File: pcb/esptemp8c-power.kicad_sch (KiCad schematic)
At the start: 27 parts, among them J4 24VAC, J5 USB_C_Receptacle_USB2.0, U2 BD9G101G, U3 AMS1117-3.3

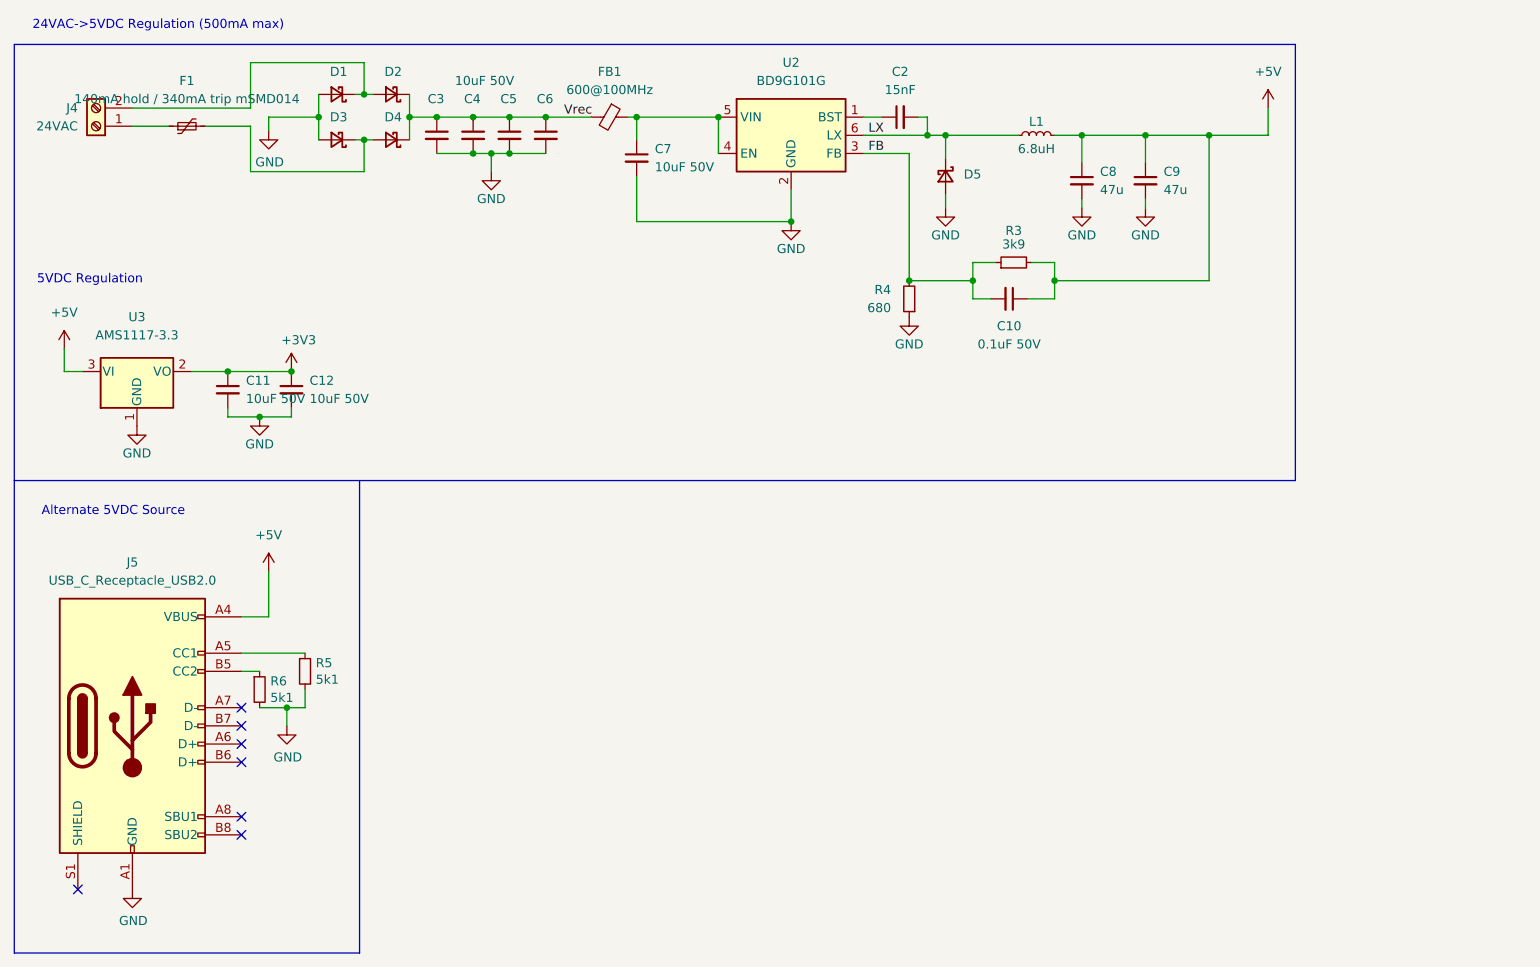
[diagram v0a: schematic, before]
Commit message: updates for v2
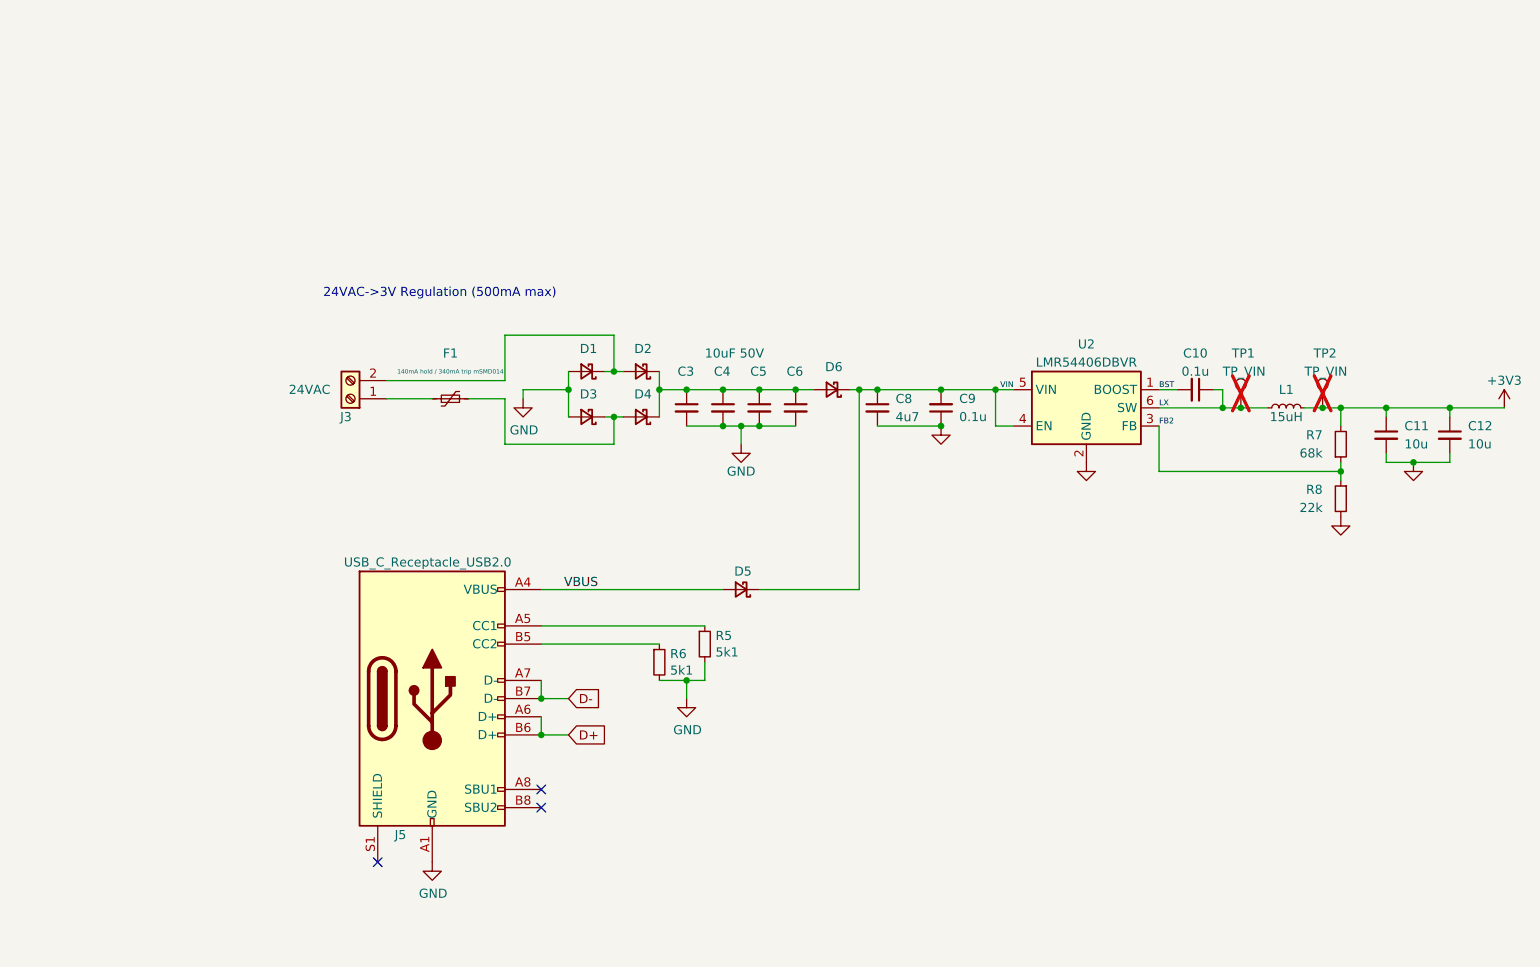
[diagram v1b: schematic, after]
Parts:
- removed C2: 15nF, Capacitor_SMD:C_0603_1608Metric, symbol Device:C_Small
- removed C7: 10uF 50V, Capacitor_SMD:C_1206_3216Metric, symbol Device:C_Small
- removed FB1: 600@100MHz, Inductor_SMD:L_0805_2012Metric, symbol Device:FerriteBead_Small
- removed J4: 24VAC, Connector_Phoenix_MSTB:PhoenixContact_MSTBA_2,5_2-G-5,08_1x02_P5.08mm_Horizontal, symbol Connector:Screw_Terminal_01x02
- removed R3: 3k9, Resistor_SMD:R_0402_1005Metric, symbol Device:R_Small
- removed R4: 680, Resistor_SMD:R_0402_1005Metric, symbol Device:R_Small
- removed U2: BD9G101G, Package_TO_SOT_SMD:SOT-23-6, symbol Regulator_Switching:AOZ1280CI
- removed U3: AMS1117-3.3, Package_TO_SOT_SMD:SOT-223-3_TabPin2, symbol Regulator_Linear:AP1117-33
- added D6: SS210, Diode_SMD:D_SMA, symbol Device:D_Schottky_Small
- added J3: 24VAC, Connector_Phoenix_MC:PhoenixContact_MC_1,5_2-G-3.81_1x02_P3.81mm_Horizontal, symbol Connector:Screw_Terminal_01x02
- added R7: 68k, Resistor_SMD:R_0402_1005Metric, symbol Device:R_Small
- added R8: 22k, Resistor_SMD:R_0402_1005Metric, symbol Device:R_Small
- added TP1, TP2: TP_VIN, Connector_PinHeader_2.54mm:PinHeader_1x01_P2.54mm_Vertical, symbol Connector:TestPoint
- added U2: LMR54406DBVR, Package_TO_SOT_SMD:TSOT-23-6, symbol Regulator_Switching:LM2840X
- C10: value 0.1uF 50V -> 0.1u
- C11, C12: value 10uF 50V -> 10u; footprint Capacitor_SMD:C_1206_3216Metric -> Capacitor_SMD:C_0805_2012Metric; LCSC C13585 -> C15850
- C8: value 47u -> 4u7; LCSC C96123 -> C29823
- C9: value 47u -> 0.1u; footprint Capacitor_SMD:C_1206_3216Metric -> Capacitor_SMD:C_0603_1608Metric; LCSC C96123 -> C14663
- D5: value SS210 -> CUS05S40.H3F; footprint Diode_SMD:D_SMA -> Diode_SMD:D_SOD-323; LCSC C14996 -> C2762696
- J5: symbol Connector:USB_C_Receptacle_USB2.0 -> Connector:USB_C_Receptacle_USB2.0_16P
- L1: value 6.8uH -> 15uH; footprint Inductor_SMD:L_Sunlord_SWPA60xxS -> Inductor_SMD:L_Sunlord_SWPA6028S; LCSC C57254 -> C83373; PN (none) -> SRN6045-150M or SWPA6045S150MT
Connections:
- net +3V3: now also L1.2, R7.2, TP2.1
- net GND: now also C9.1, R8.2, U2.2 (GND); no longer C9.2, D5.2 (A)
- net LX: now also C10.1, TP1.1, U2.6 (SW); no longer D5.1 (K)
- net D+: now reaches J5.A6 (D+)
- net D+: now also J5.B6 (D+)
- net D-: now reaches J5.A7 (D-)
- net D-: now also J5.B7 (D-)
- net at F1.1: now also J3.1 (Pin_1)
- net at D1.1 (K), D2.2 (A): now also J3.2 (Pin_2)
- net +5V renamed VBUS
- net VBUS: now also D5.2 (A); no longer C10.1, C8.1, C9.1, L1.2
- net FB renamed BST
- net BST: now also U2.1 (BOOST)
- net Vrec: no longer names the net of C3.1, C4.1, C5.1, C6.1, D2.1 (K), D4.1 (K)
- net Vrec: now also D6.2 (A)
- new net FB2: R7.1, R8.1, U2.3 (FB)
- new net VIN: C8.1, C9.2, D5.1 (K), D6.1 (K), U2.4 (EN), U2.5 (VIN)
- no-connect marks 7 -> 3
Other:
- note added: "24VAC->3V Regulation (500mA max)"
- note removed: "24VAC->5VDC Regulation (500mA max)"
- note removed: "5VDC Regulation"
- note removed: "Alternate 5VDC Source"
- moved on the sheet: C3, C4, C5, C6, D1, D2, D3, D4, F1, J5, R5, R6
